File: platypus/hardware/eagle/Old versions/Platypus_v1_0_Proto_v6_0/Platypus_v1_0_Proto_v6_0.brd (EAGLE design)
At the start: 25.1 x 35.5 mm, 27 parts, among them J1 EDISON_CONNECTOR_FULLMOUNTING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, U1 MPU-9250, U2 TXB0108, U3 MAX17043, X3 Power TP, X4 I2C TP, X5 Display TP

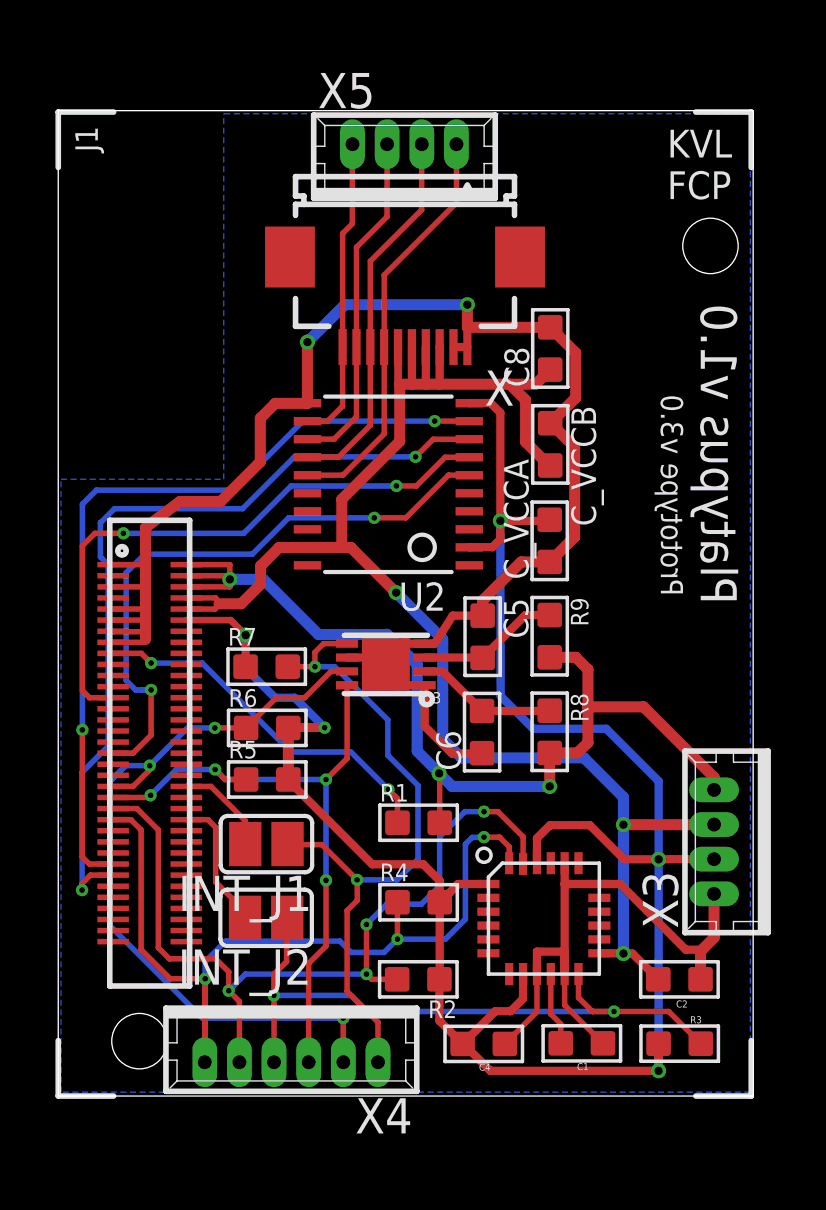
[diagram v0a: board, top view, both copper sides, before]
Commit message: updated platypus hardware folder
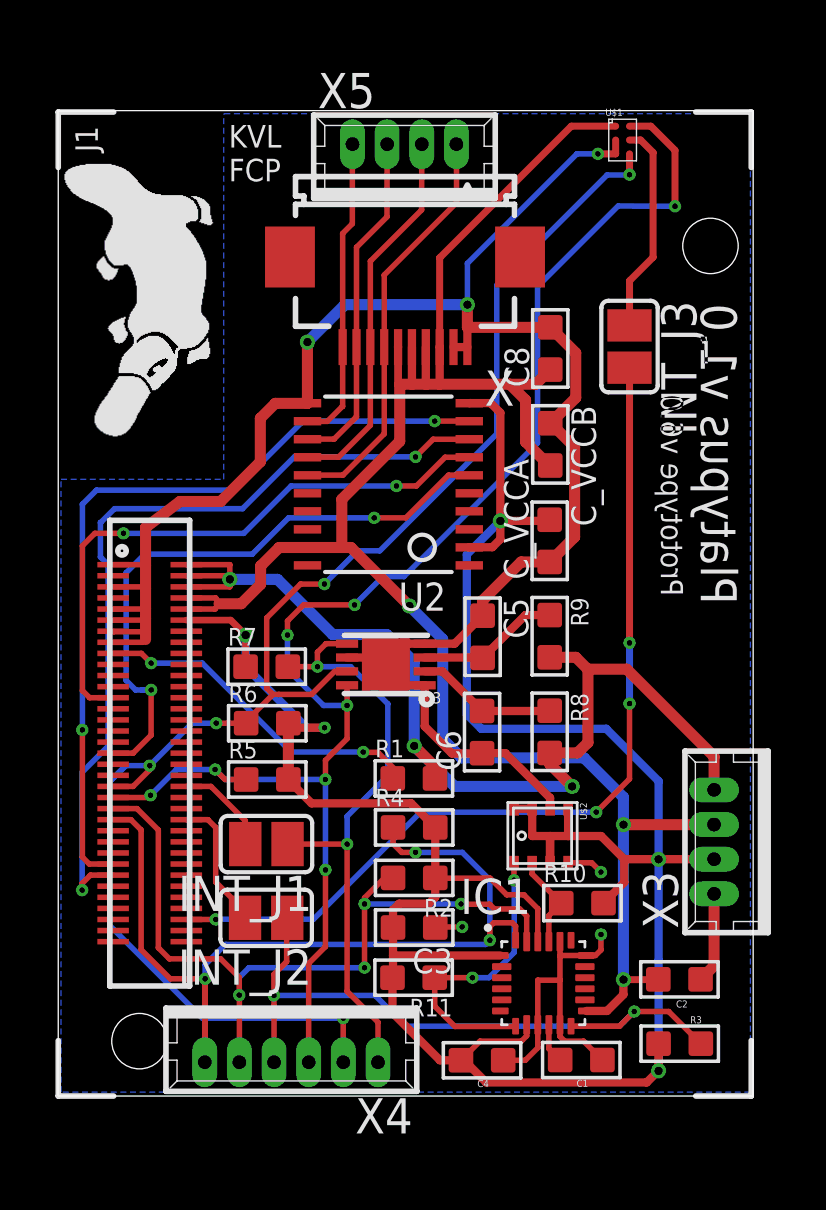
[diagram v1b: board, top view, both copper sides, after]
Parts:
- removed U1: MPU-9250, template:LGA-24
- added C3: 100nF, Discrete:C0603
- added IC1: MPU-9250, invensense:QFN24-SMALL
- added INT_J3: (no value), jumper:SJ
- added R10, R11: 4.7k, Discrete:R0603
- added U$1: TSL2584TSV6-XFBGA, TSL2584TSV:6-XFBGA
- added U$2: BME280LGA-8, BME280:LGA-8
- U2: value TXB0108 -> TXS0108E
- moved R2 3.66 mm to (85.2, 19.3)
- moved R4 2.70 mm to (85.2, 21.1)
- moved R1 1.61 mm to (85.2, 22.9)
- moved C1 0.60 mm to (91.3, 12.7)
- moved C4 0.59 mm to (87.7, 12.7)
- moved R6 0.17 mm to (79.9, 24.9)
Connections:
- new net ALS_INT: INT_J3.1, U$1.P$5
- new net AUX_CL: IC1.7, R11.1, U$2.P$4
- new net AUX_DA: IC1.21, R10.1, U$2.P$3
- net 1.8V: now also C3.2, IC1.1, IC1.22, IC1.8, R10.2, R11.2, U$2.P$2, U$2.P$5, U$2.P$6, U$2.P$8; no longer U1.1, U1.22, U1.8
- net 3.3V: now also IC1.13, U$1.P$1; no longer U1.13
- net GND: now also C3.1, IC1.11, IC1.18, IC1.20, IC1.9, U$1.P$2, U$1.P$3, U$2.P$1, U$2.P$7; no longer U1.11, U1.18, U1.20, U1.9
- net GP19_I2C_1_SCL: now also U$1.P$4
- net GP20_I2C_1_SDA: now also U$1.P$6
- net GP27_I2C_6_SCL: now also IC1.23; no longer U1.23
- net GP28_I2C_6_SDA: now also IC1.24; no longer U1.24
- net GP80_SD_0_DAT0: now also INT_J3.2
- net IMU_INT: now also IC1.12; no longer U1.12
- net N$5: now also IC1.10; no longer U1.10
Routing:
- net GP80_SD_0_DAT0: track 0.00 -> 32.9 mm, vias 0 -> 4
- net GP20_I2C_1_SDA: track 23.7 -> 55.6 mm, vias 4 -> 8
- net GP19_I2C_1_SCL: track 29.3 -> 55.9 mm, vias 3 -> 5
- net 3.3V: track 57.1 -> 70.5 mm
- net AUX_CL: track 0.00 -> 10.8 mm, vias 0 -> 2
- net 1.8V: track 90.3 -> 100.2 mm
- net GND: track 80.4 -> 88.6 mm, vias 2 -> 6
- net ALS_INT: track 0.00 -> 7.63 mm
- net AUX_DA: track 0.00 -> 3.47 mm
- net GP28_I2C_6_SDA: track 31.9 -> 34.4 mm
- net BAT_ALERT: track 24.4 -> 22.1 mm
- net VSYS: track 36.9 -> 38.6 mm
- net GP27_I2C_6_SCL: track 30.4 -> 28.8 mm
- net N$5: track 2.65 -> 1.44 mm
- net PWRBTN#: track 13.3 -> 12.7 mm
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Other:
- board text added: "9DOF IMU"
- board text added: "Ambient Light Sensor"
- board text added: "BME 280"
- board text added: "C3 100nF"
- board text added: "J_ALS"
- board text added: "MPU 9255"
- board text added: "Pressure Humidity Temperature Sensor"
- board text added: "Prototype v6.0"
- board text added: "R10 4k7"
- board text added: "R11 4k7"
- board text added: "TSL2584TSV"
- board text added: "TXS0108E"
- board text removed: "MPU 9250"
- board text removed: "Prototype v3.0"
- board text removed: "TXB0108"
